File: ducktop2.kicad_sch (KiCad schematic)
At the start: 0 parts

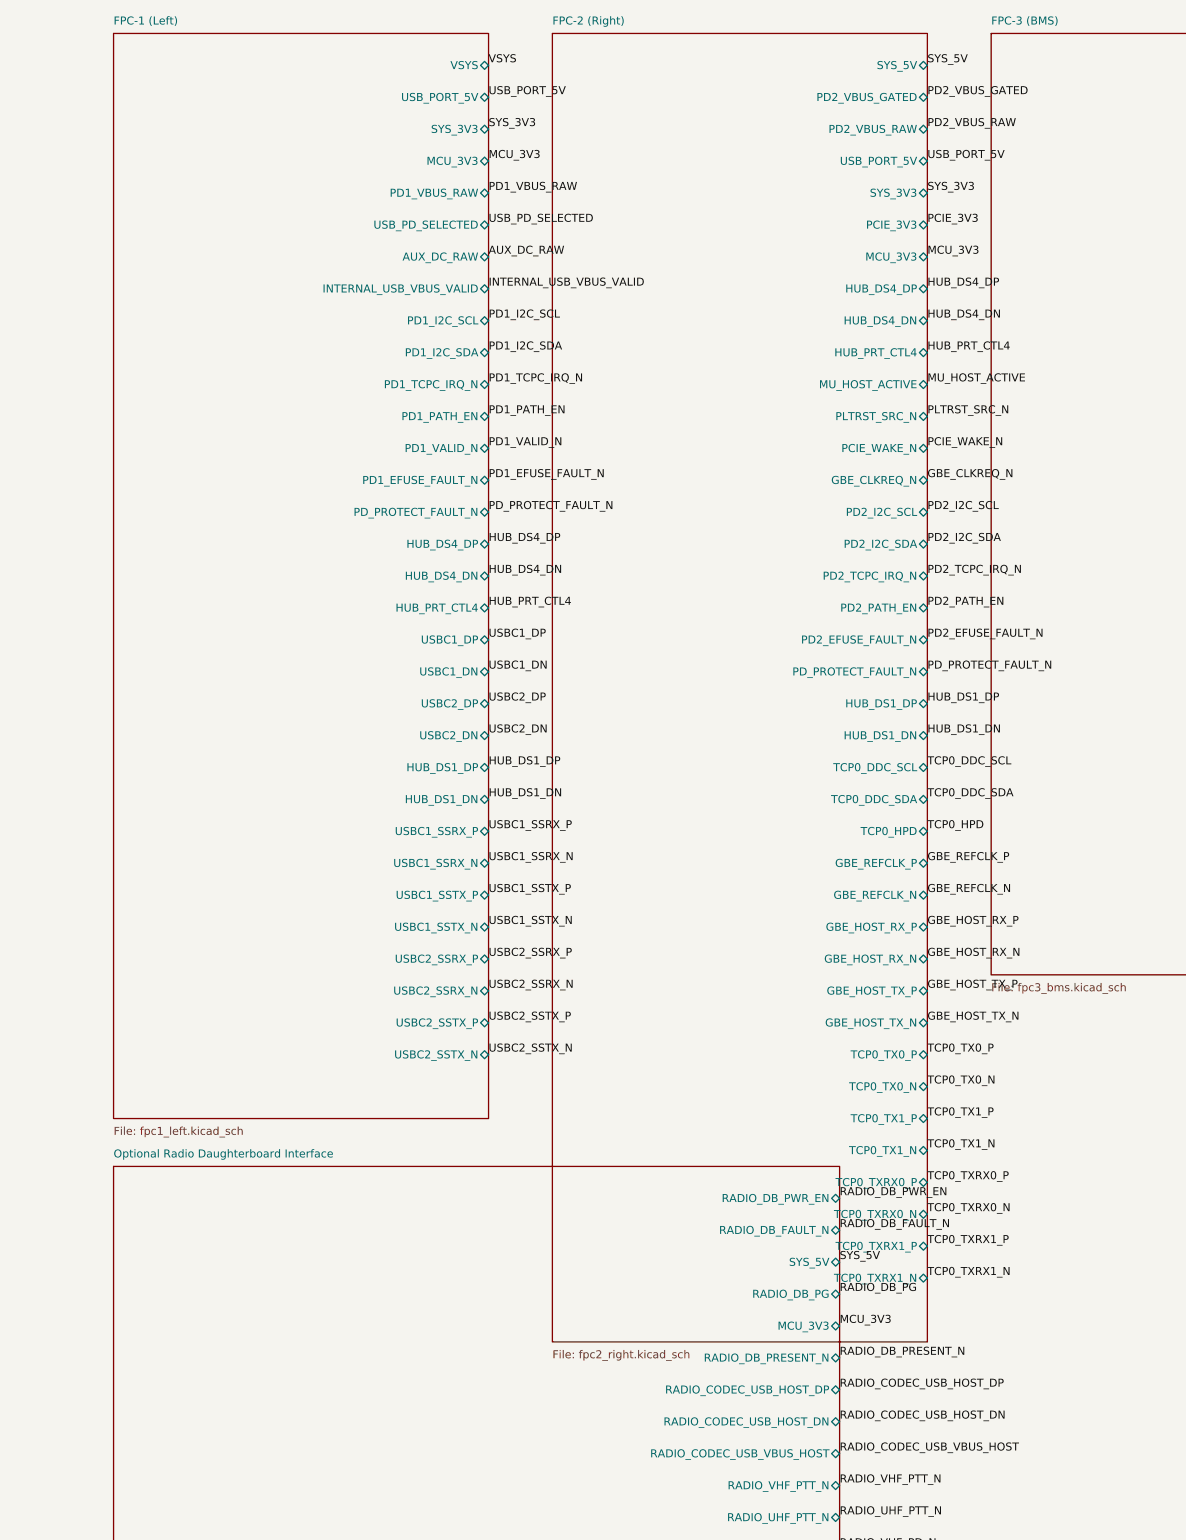
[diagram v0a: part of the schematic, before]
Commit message: fix the center layout and more board issues
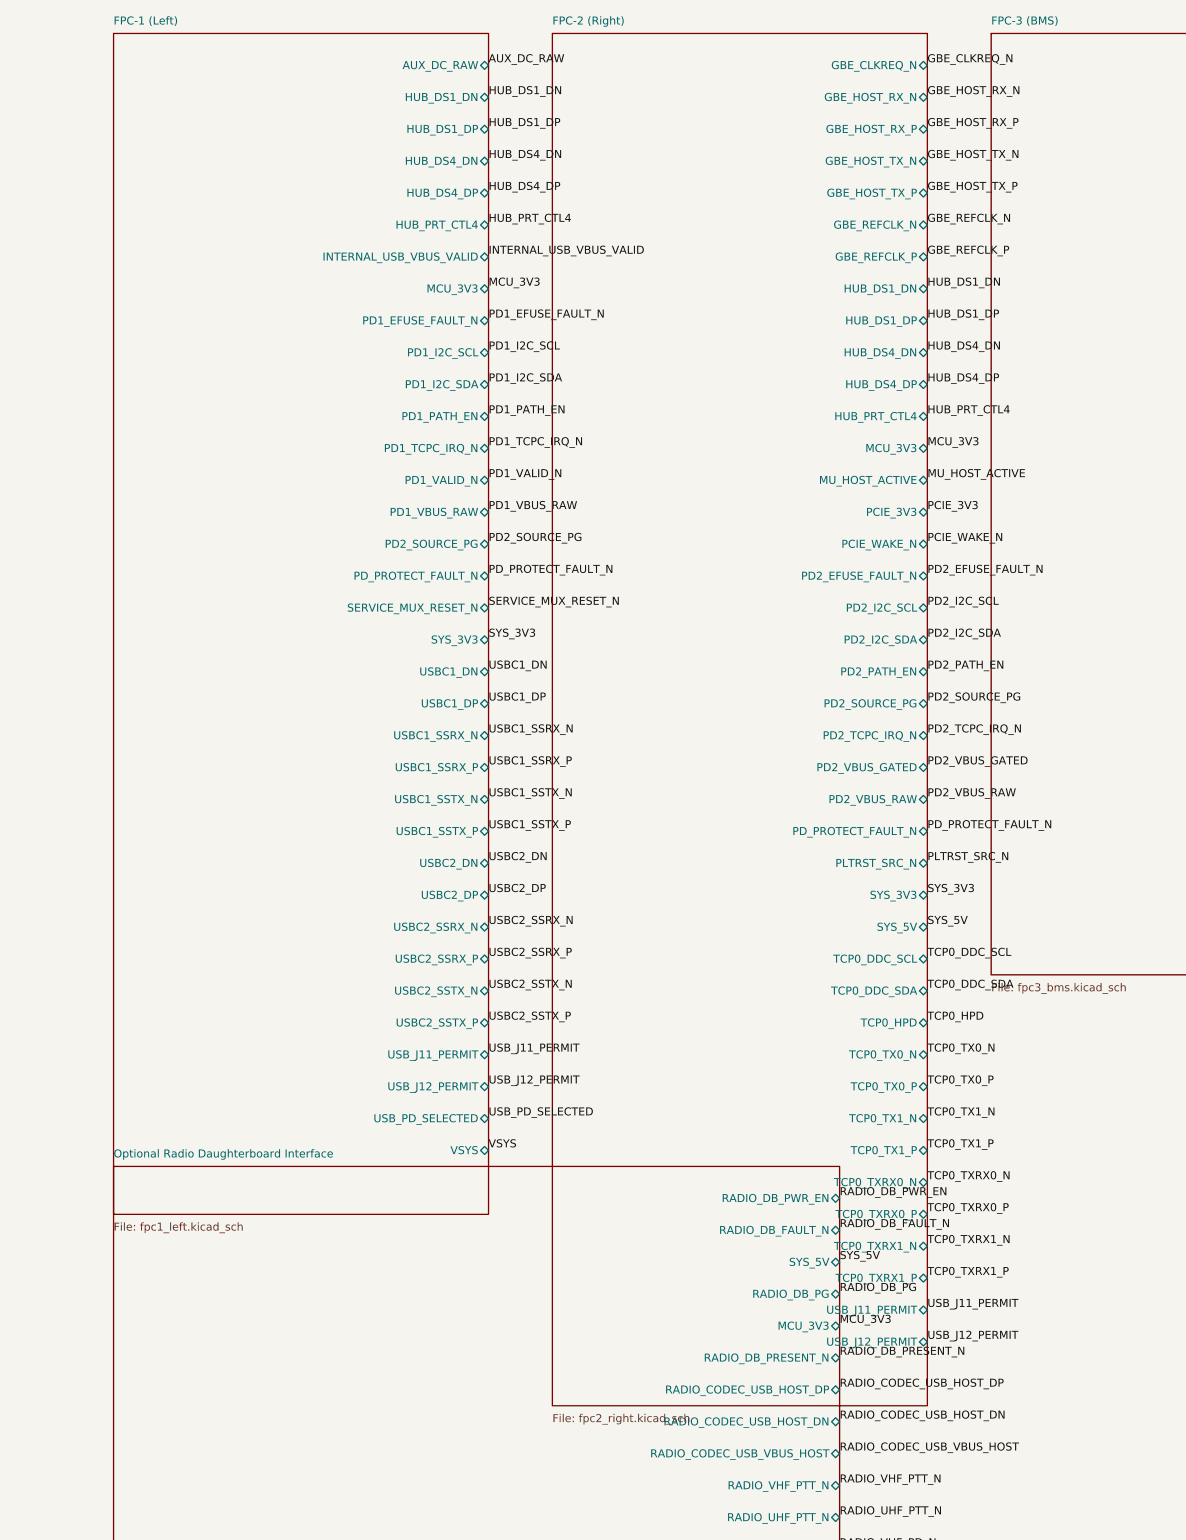
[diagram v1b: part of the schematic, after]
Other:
- sheet FPC-1 (Left) ports: added PD2_SOURCE_PG, SERVICE_MUX_RESET_N, USB_J11_PERMIT, USB_J12_PERMIT; removed USB_PORT_5V
- sheet FPC-2 (Right) ports: added PD2_SOURCE_PG, USB_J11_PERMIT, USB_J12_PERMIT; removed USB_PORT_5V
